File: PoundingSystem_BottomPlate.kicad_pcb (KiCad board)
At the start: 4 copper layers, 184.2 x 223.8 mm, 5 parts

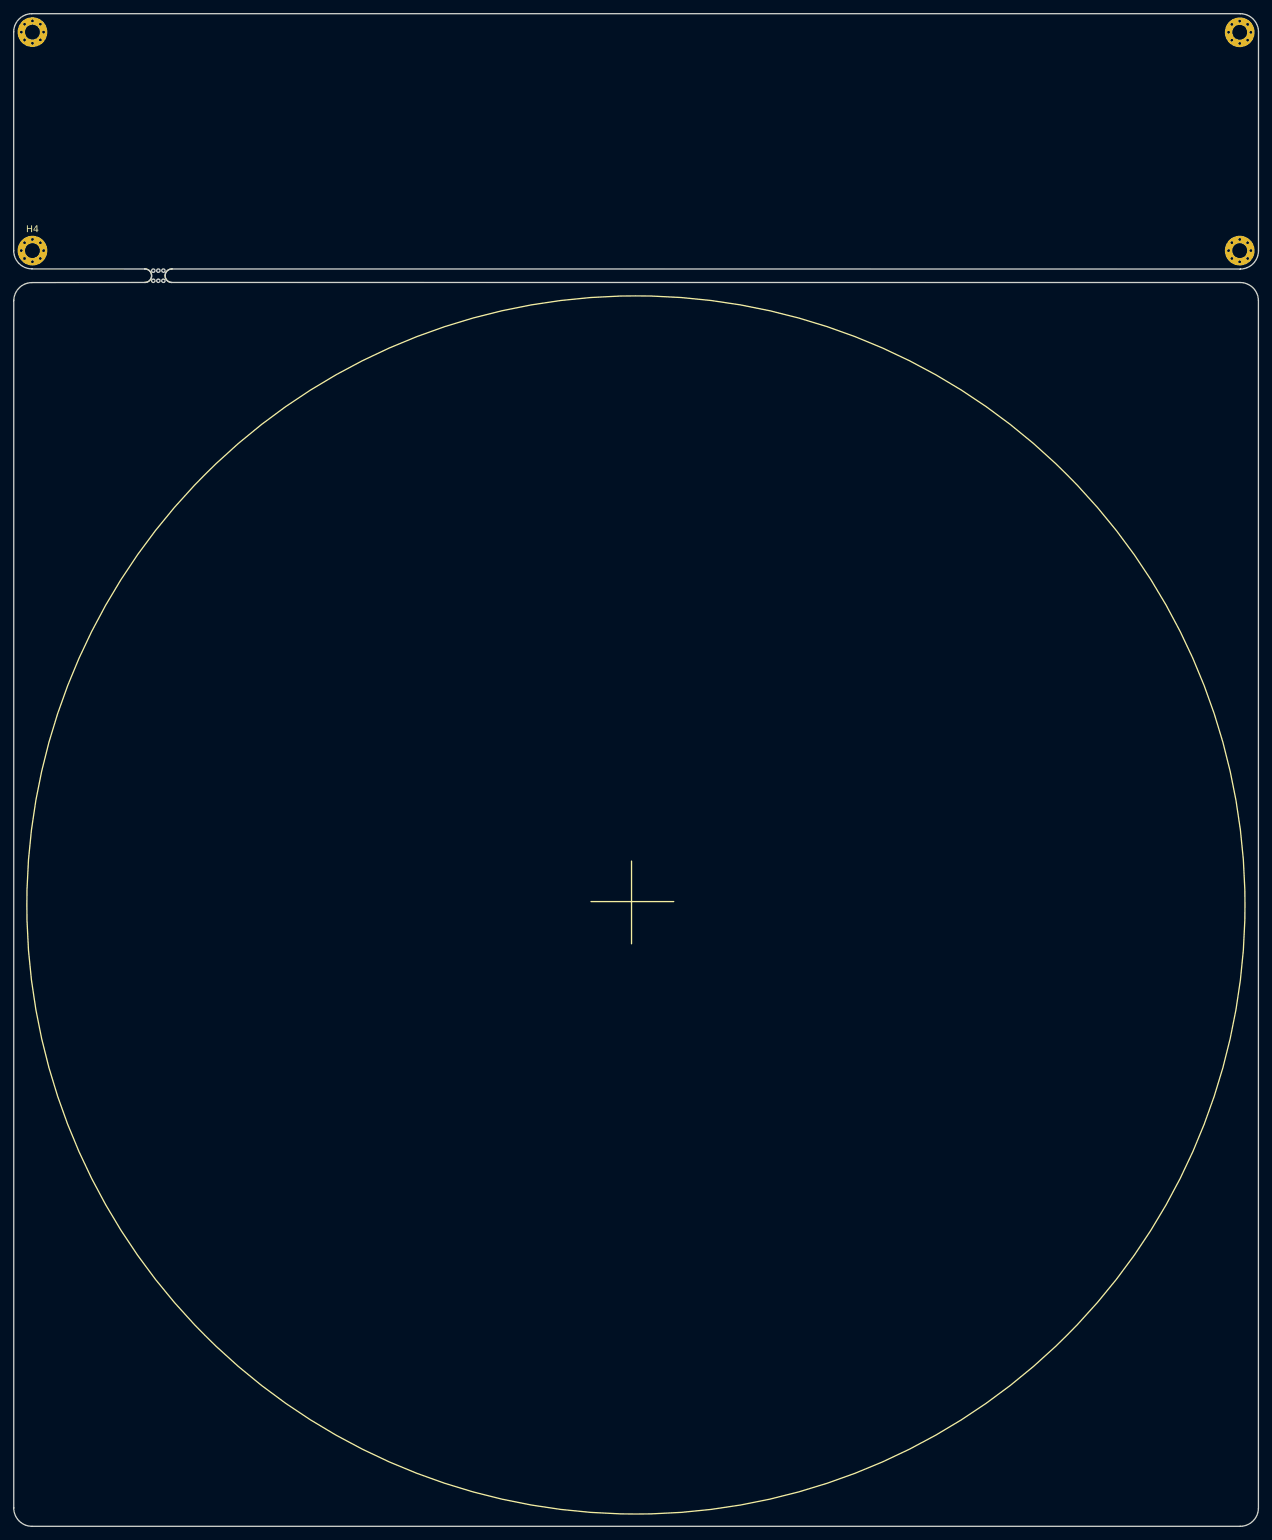
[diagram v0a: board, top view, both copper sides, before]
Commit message: h7 version;
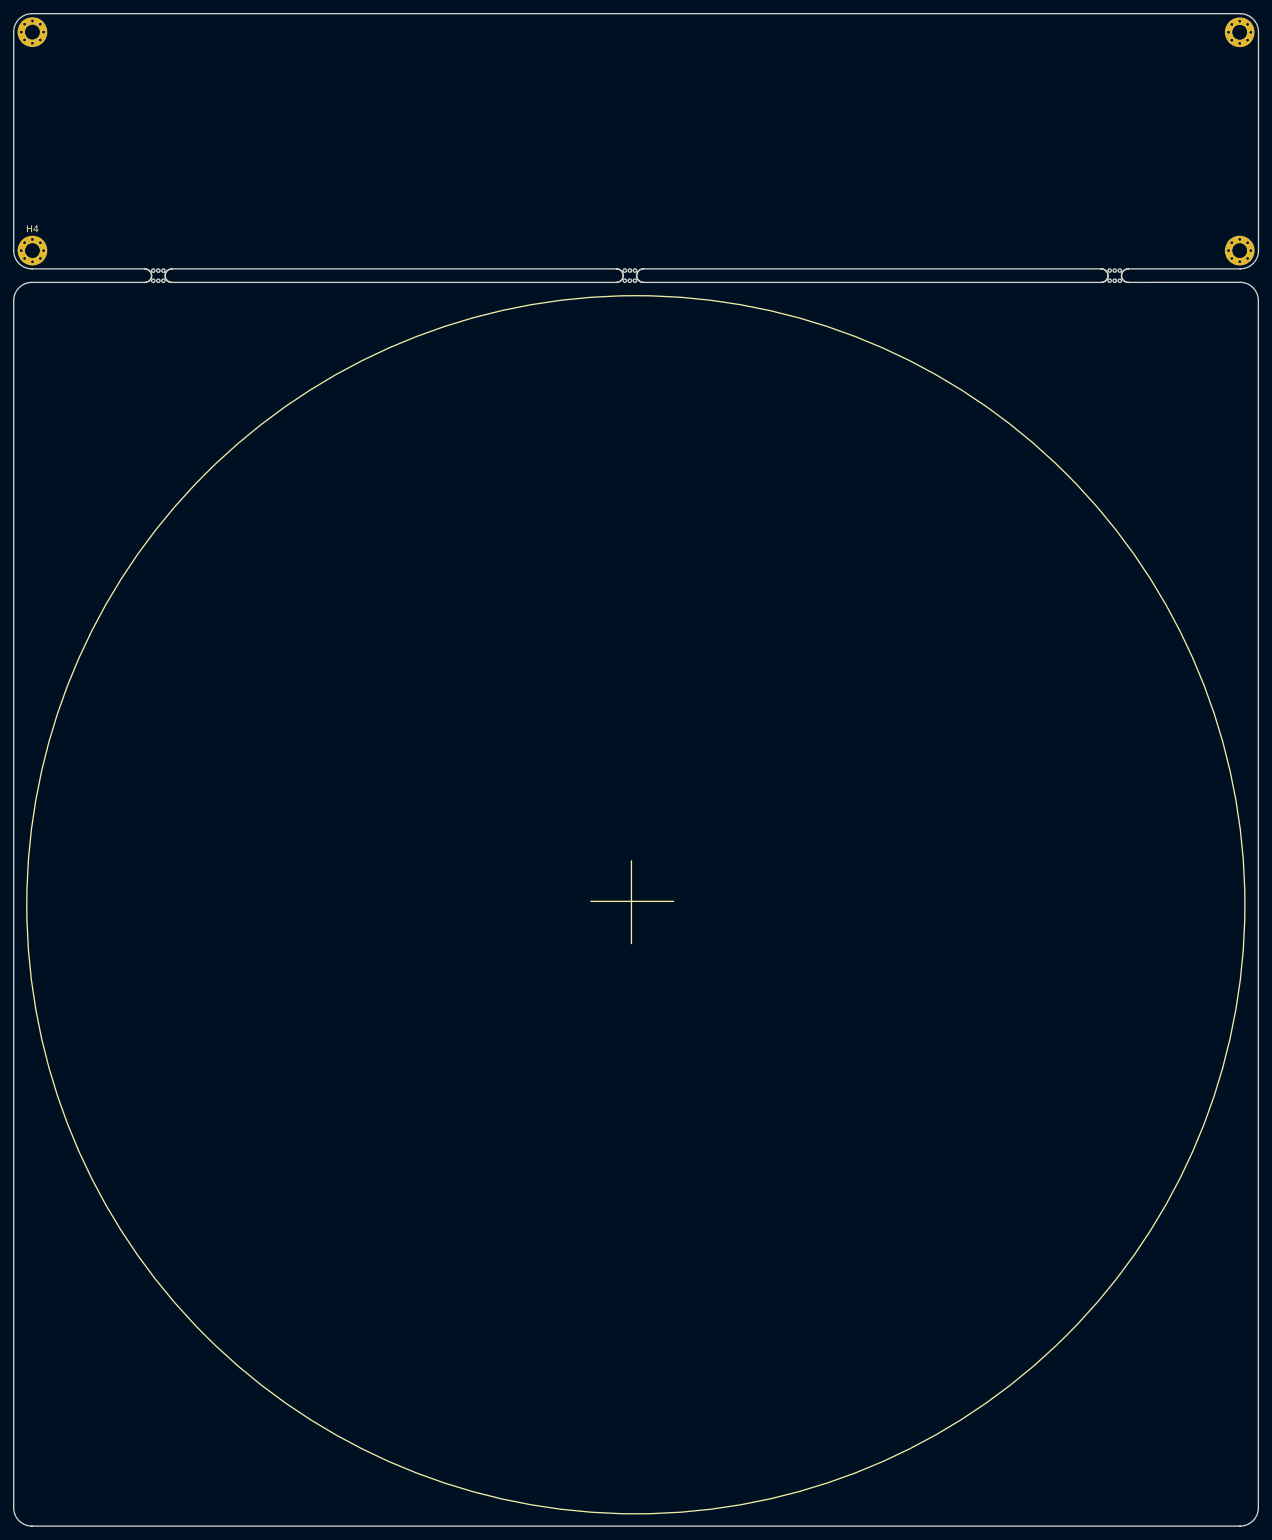
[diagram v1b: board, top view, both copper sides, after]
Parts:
- added mouse-bite-2mm-slot: VAL**, Panelization:mouse-bite-2mm-slot, F.Cu at (135.3, 45.9)
- added mouse-bite-2mm-slot: VAL**, Panelization:mouse-bite-2mm-slot, F.Cu at (207.0, 45.9)
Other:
- board size 184.2 x 223.8 mm -> 184.2 x 223.7 mm

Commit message: production: generate production files
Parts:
- added G***: LOGO, Camo:Layer1, F.Cu at (136.1, 119.6)
- added H1: MountingHole_Pad, MountingHole:MountingHole_2.2mm_M2_Pad_Via, F.Cu at (225.5, 228.1)
- added H1: MountingHole_Pad, MountingHole:MountingHole_2.2mm_M2_Pad_Via, F.Cu at (225.5, 49.7)
- added H4: MountingHole_Pad, MountingHole:MountingHole_2.2mm_M2_Pad_Via, F.Cu at (46.9, 228.1)
- added H4: MountingHole_Pad, MountingHole:MountingHole_2.2mm_M2_Pad_Via, F.Cu at (46.9, 49.7)
- added REF**: LED_D3.0mm, LED_THT:LED_D3.0mm, B.Cu at (134.2, 138.5)
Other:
- board text removed: "TO DO: - Power Switch - Components and wiring for audio jacks"
